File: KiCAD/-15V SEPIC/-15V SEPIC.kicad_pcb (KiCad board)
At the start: 4 copper layers, 24 x 30 mm, 21 parts, among them J1 Conn_01x04_Pin, U1 LT3579

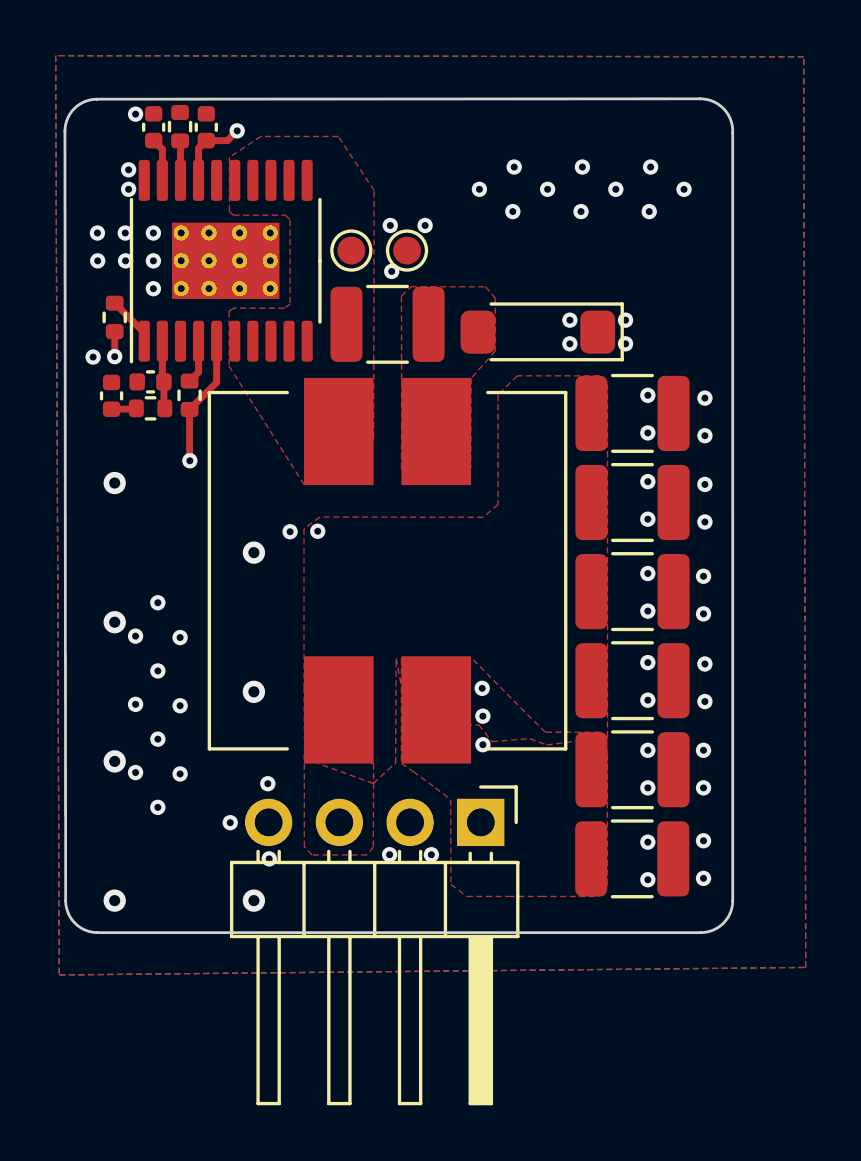
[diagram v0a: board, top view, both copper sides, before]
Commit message: kicad sepic update
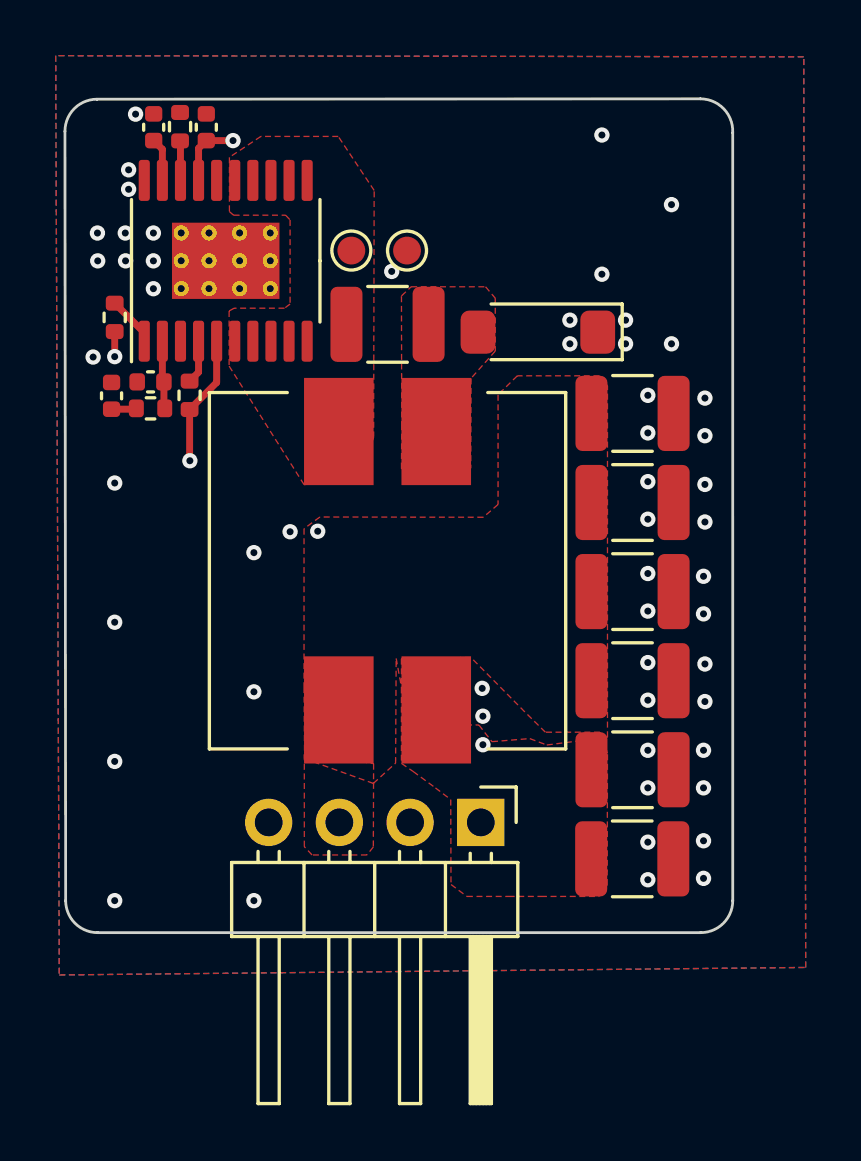
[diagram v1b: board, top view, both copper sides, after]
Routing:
- net GND: vias 75 -> 52
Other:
- board text added: "AUDIO DSP"
- board text added: "JLCJLCJLCJLC"
- board text added: "SEPIC -15V"
